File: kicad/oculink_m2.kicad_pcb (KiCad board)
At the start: 4 copper layers, 100.5 x 113.2 mm, 18 parts, among them J1 G14A42121B12HR

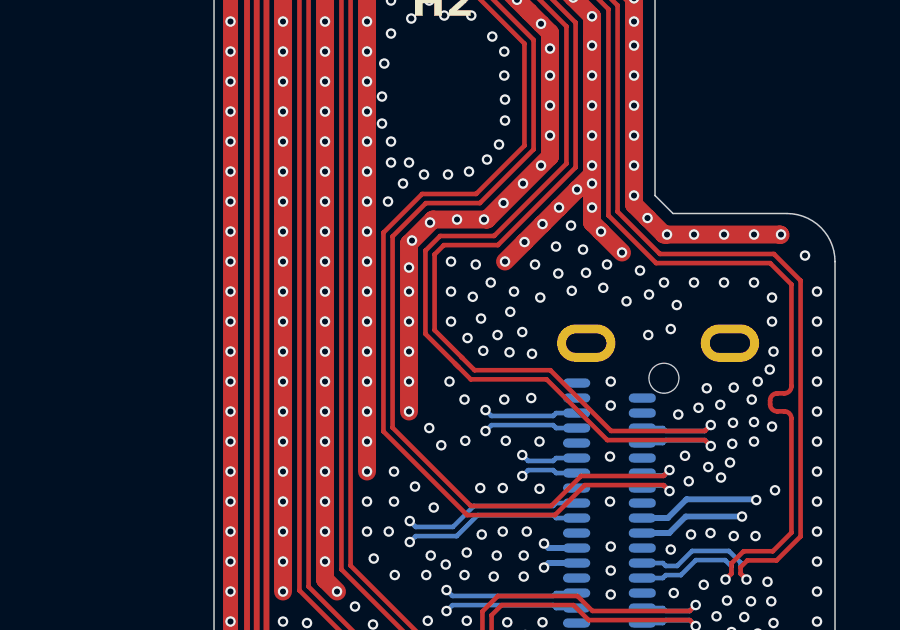
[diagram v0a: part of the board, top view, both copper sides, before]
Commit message: Added design rule check for 85ohm impedance matched differential pairs
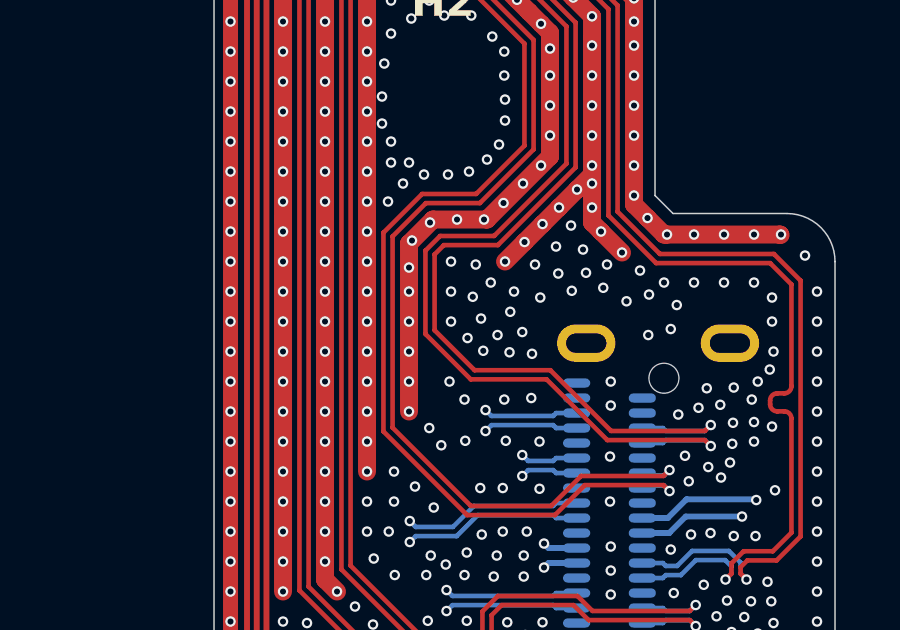
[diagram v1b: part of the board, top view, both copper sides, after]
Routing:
- net SMB-: track 158.5 -> 157.6 mm

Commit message: Fixed up diff pair custom rules
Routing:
- net SMB-: track 157.6 -> 158.5 mm
